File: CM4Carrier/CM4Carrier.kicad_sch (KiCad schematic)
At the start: 0 parts

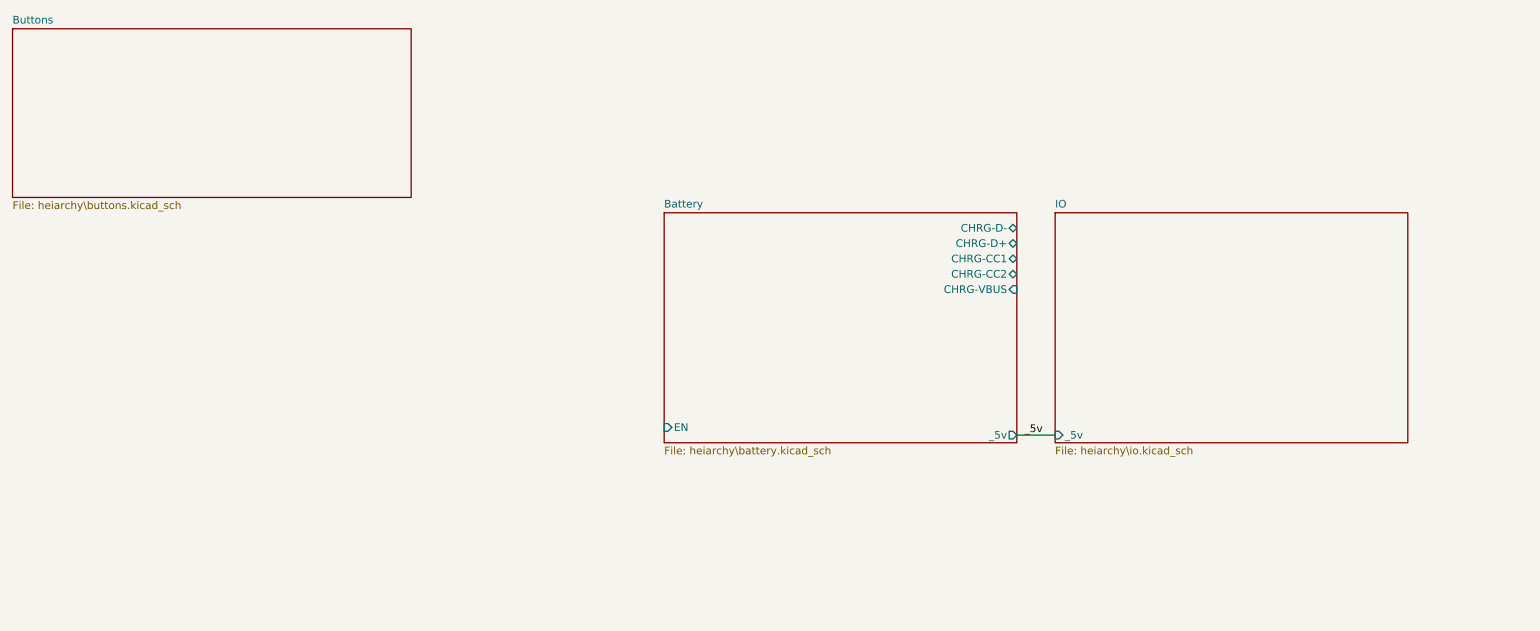
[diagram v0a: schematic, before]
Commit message: Additions
- Fixed gitignore (Backups)
- Work on buttons
- Work on ADC for JOYSTICK
- Work on some other stuff
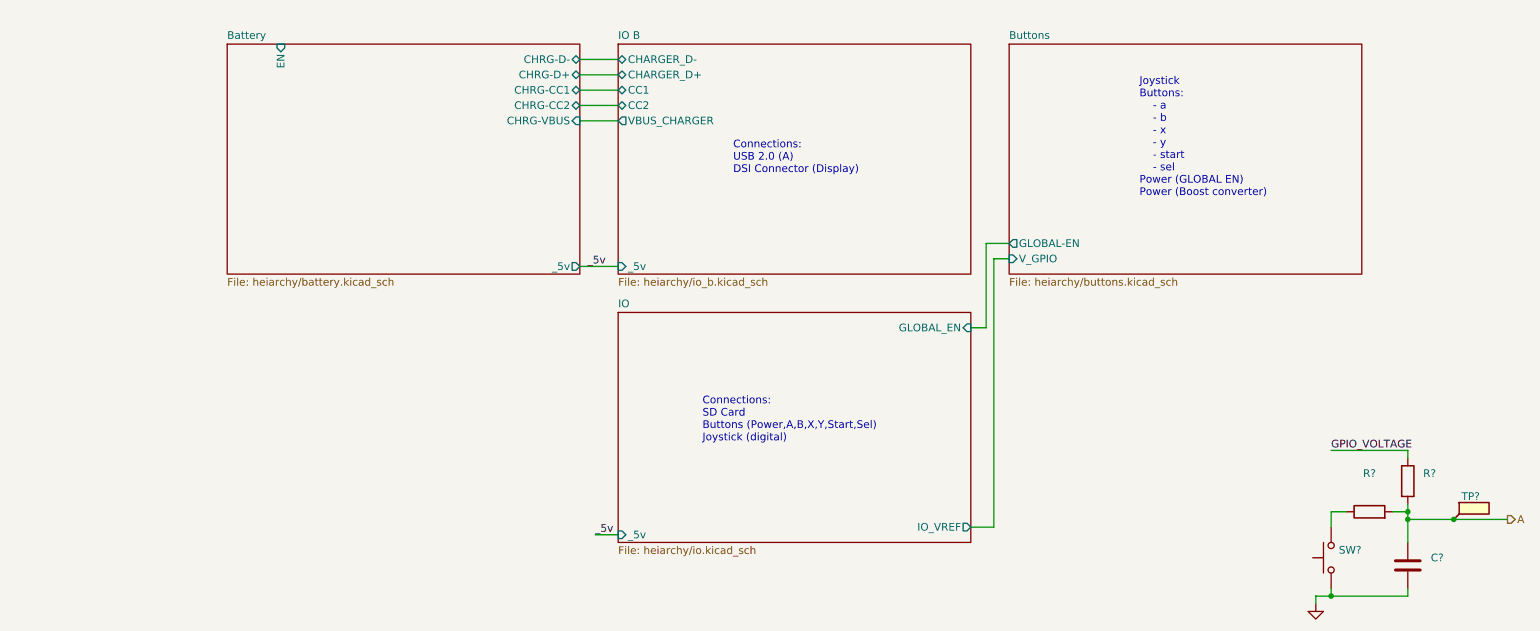
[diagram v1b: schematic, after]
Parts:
- added C?: (no value), symbol Device:C
- added R? (x2): (no value), symbol Device:R
- added SW?: (no value), symbol Switch:SW_Push
- added TP?: ~, symbol Connector:TestPoint_Flag
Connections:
- new net: R?.1, SW?.2
- new net A: C?.1, R?.2, R?.2, TP?.1
- new net GND: C?.2, SW?.1
- new net GPIO_VOLTAGE: R?.1
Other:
- added sheet IO B (heiarchy/io_b.kicad_sch)
- sheet Battery: file heiarchy\battery.kicad_sch -> heiarchy/battery.kicad_sch
- sheet Buttons: file heiarchy\buttons.kicad_sch -> heiarchy/buttons.kicad_sch
- sheet Buttons ports: added GLOBAL-EN, V_GPIO; removed none
- sheet IO: file heiarchy\io.kicad_sch -> heiarchy/io.kicad_sch
- sheet IO ports: added GLOBAL_EN, IO_VREF; removed none
- note added: "Connections: SD Card Buttons (Power,A,B,X,Y,Start,Sel) Joystick (digital)"
- note added: "Connections: USB 2.0 (A) DSI Connector (Display)"
- note added: "Joystick Buttons: - a - b - x - y - start - sel Power (GLOBAL EN) Power (Boost converter)"
